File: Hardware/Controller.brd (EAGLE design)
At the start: 100 x 80 mm, 0 parts

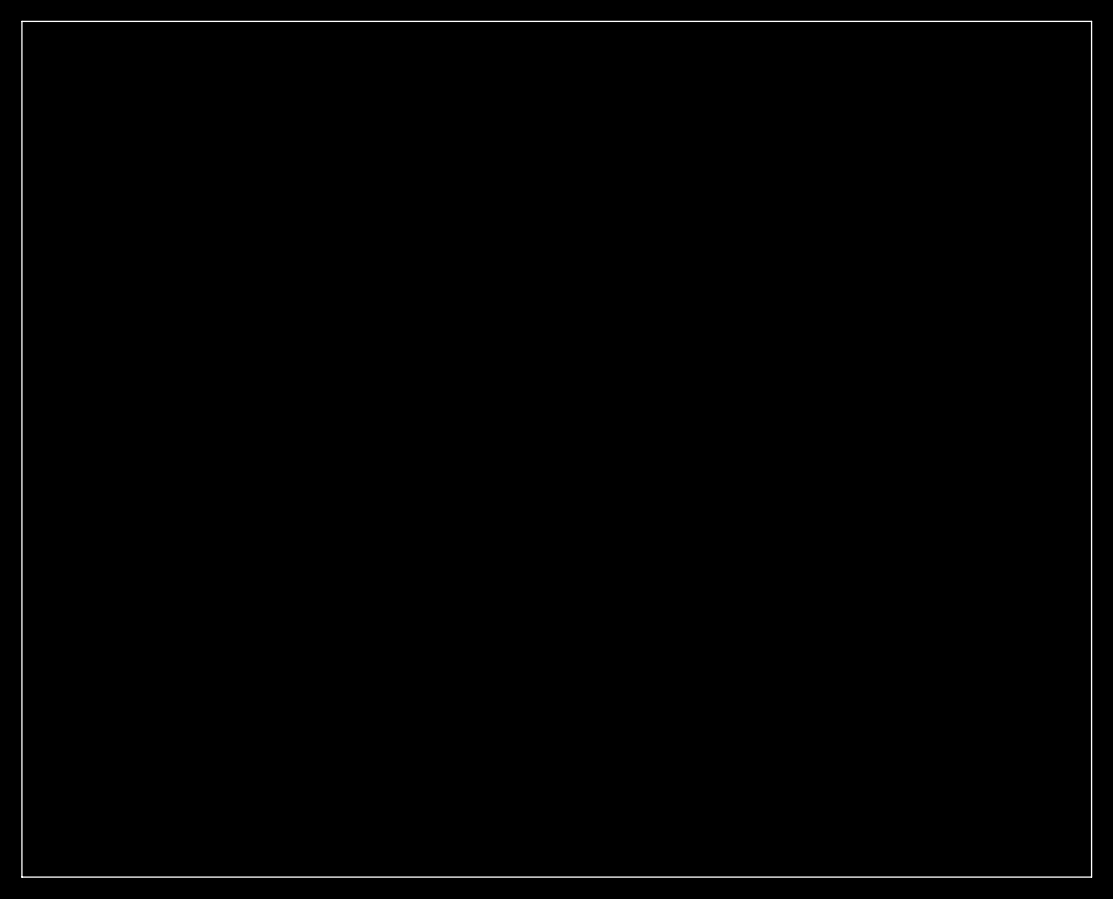
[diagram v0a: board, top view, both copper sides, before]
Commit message: controller board draft 1
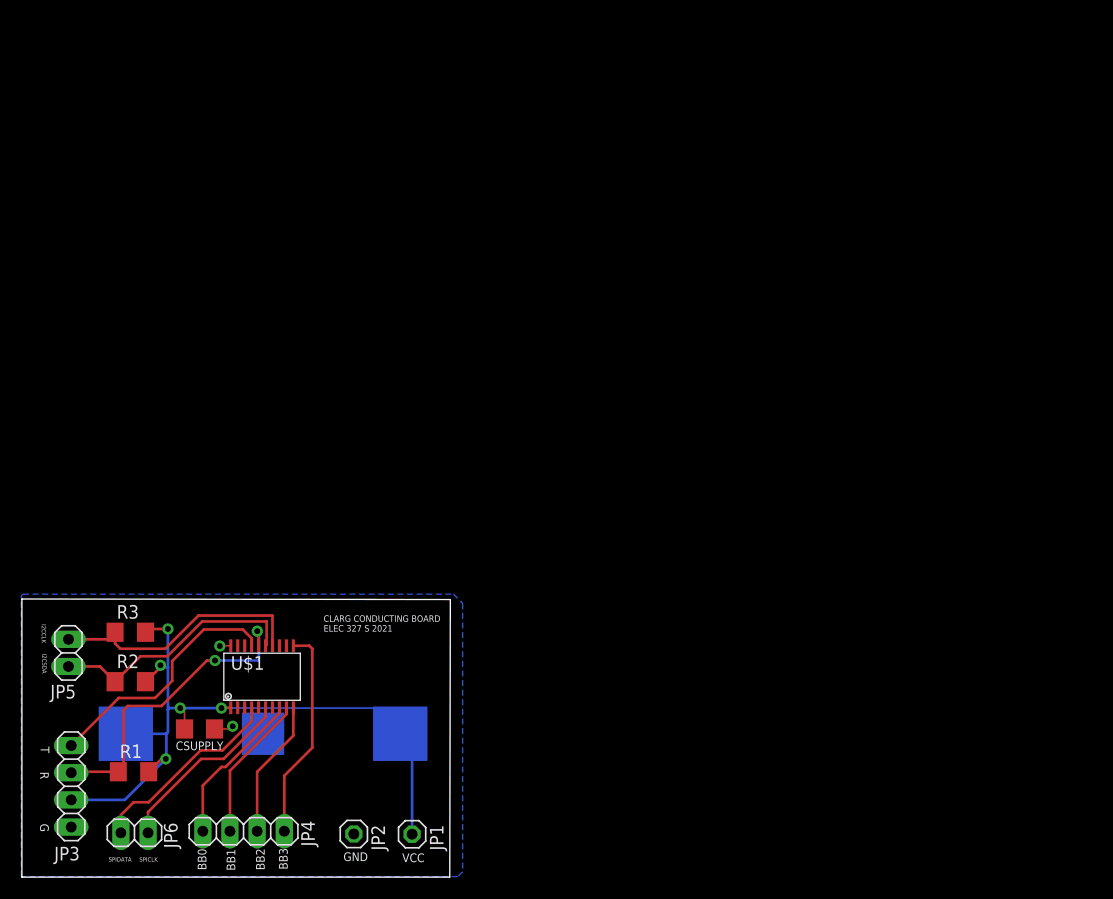
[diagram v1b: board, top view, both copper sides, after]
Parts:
- added CSUPPLY: (no value), rcl:C1206
- added JP1, JP2: (no value), pinhead:1X01
- added JP3, JP4: (no value), pinhead:1X04
- added JP5, JP6: (no value), pinhead:1X02
- added R1, R2, R3: (no value), rcl:R1206
- added U$1: MSP430G2XX3TSSOP, givenELEC327:PW20
- added U$2: 3002BATTERY, Personal:3002BATTERY
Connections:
- new net BB0: JP4.1, U$1.8
- new net BB1: JP4.2, U$1.9
- new net BB2: JP4.3, U$1.10
- new net BB3: JP4.4, U$1.11
- new net GND: CSUPPLY.2, JP2.1, JP3.1, U$1.20, U$2.P$1
- new net I2CCLK: JP5.2, R3.1, U$1.14
- new net I2CSDA: JP5.1, R2.1, U$1.15
- new net RST/SBWTDIO: JP3.3, R1.1, U$1.16
- new net SPICLK: JP6.2, U$1.6
- new net SPIDATA: JP6.1, U$1.4
- new net TEST/SBWTCK: JP3.4, U$1.17
- new net VCC: CSUPPLY.1, JP1.1, JP3.2, R1.2, R2.2, R3.2, U$1.1, U$2.P$2, U$2.P$3
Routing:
- net VCC: track 0.00 -> 69.4 mm, vias 0 -> 5
- net RST/SBWTDIO: track 0.00 -> 29.2 mm, vias 0 -> 2
- net I2CCLK: track 0.00 -> 24.7 mm
- net I2CSDA: track 0.00 -> 23.8 mm
- net TEST/SBWTCK: track 0.00 -> 23.5 mm
- net BB3: track 0.00 -> 20.0 mm
- net SPIDATA: track 0.00 -> 18.8 mm
- net SPICLK: track 0.00 -> 17.5 mm
- net BB0: track 0.00 -> 14.7 mm
- net BB1: track 0.00 -> 13.7 mm
- net BB2: track 0.00 -> 12.9 mm
- net GND: track 0.00 -> 2.84 mm, vias 0 -> 2
- added copper zone on layer 16, net GND
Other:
- board size 100 x 80 mm -> 40 x 26 mm
- board text added: "BB0"
- board text added: "BB1"
- board text added: "BB2"
- board text added: "BB3"
- board text added: "CLARG CONDUCTING BOARD ELEC 327 S 2021"
- board text added: "G"
- board text added: "GND"
- board text added: "I2CCLK"
- board text added: "I2CSDA"
- board text added: "R"
- board text added: "SPICLK"
- board text added: "SPIDATA"
- board text added: "T"
- board text added: "V"
- board text added: "VCC"
